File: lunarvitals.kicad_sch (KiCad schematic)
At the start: 29 parts, among them J1 MLX90614, J2 MAX30102, J3 SEN11574, J4 ConductiveCord, U1 NRF52840-DONGLE, U2 BMP280, U3 AP2112K-3.3, U5 MPU-6050

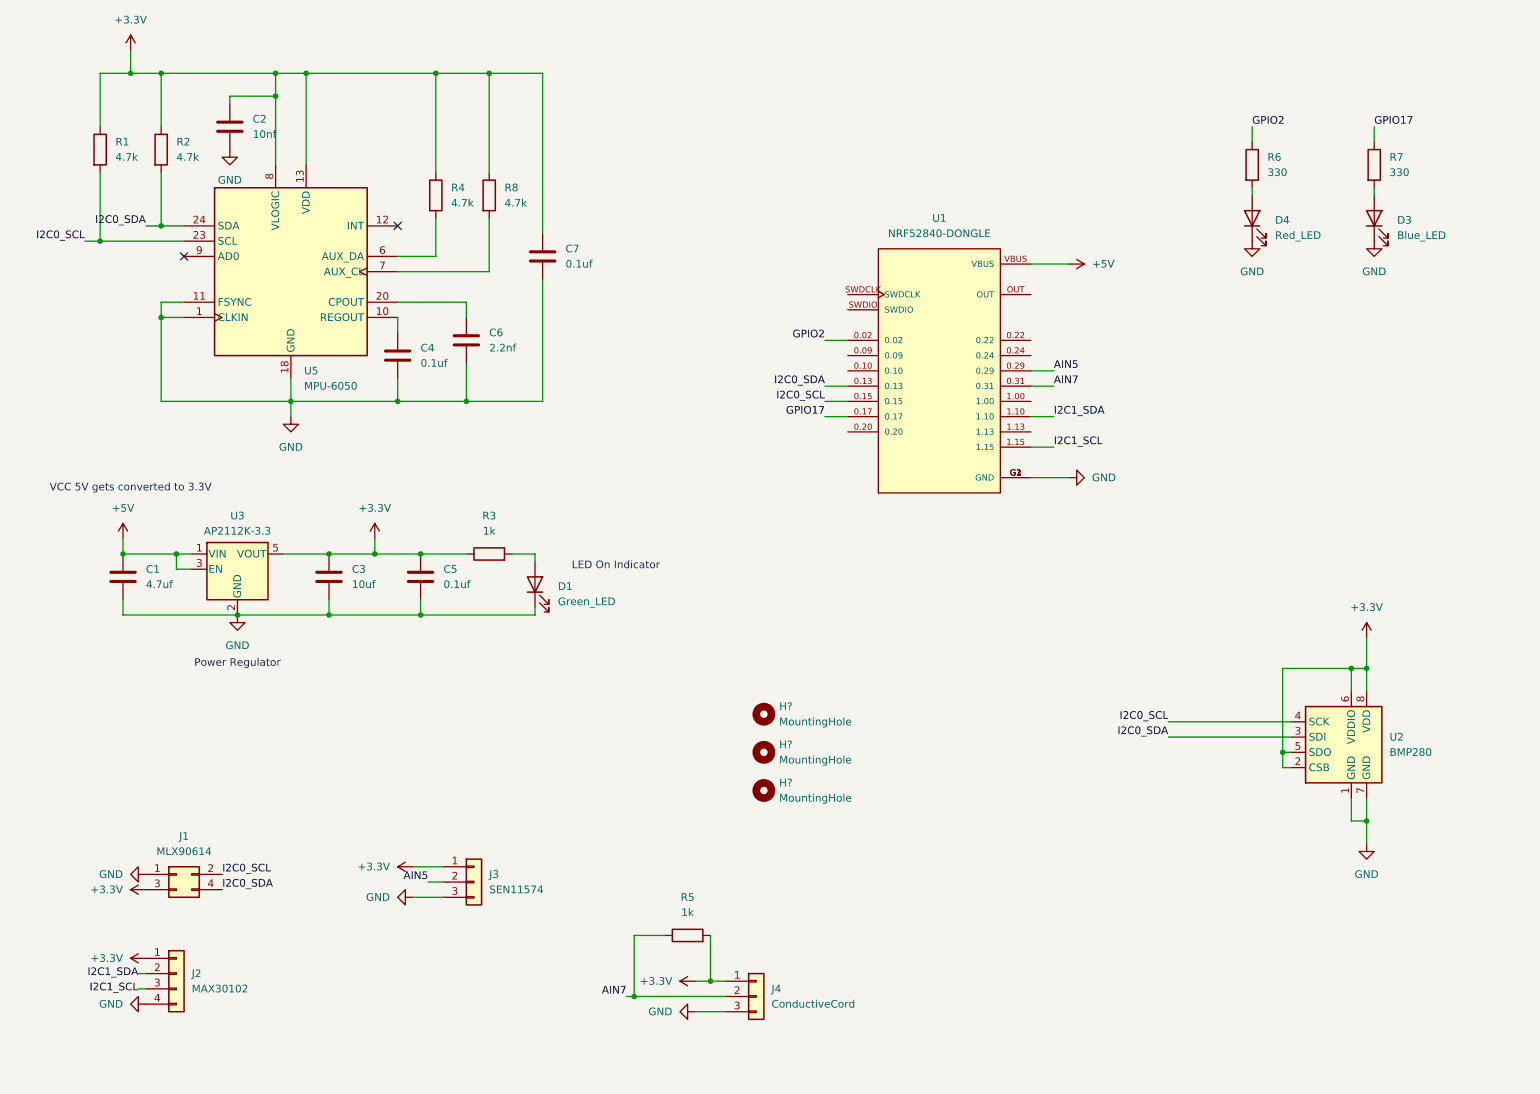
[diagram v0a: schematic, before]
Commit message: PCB Updates
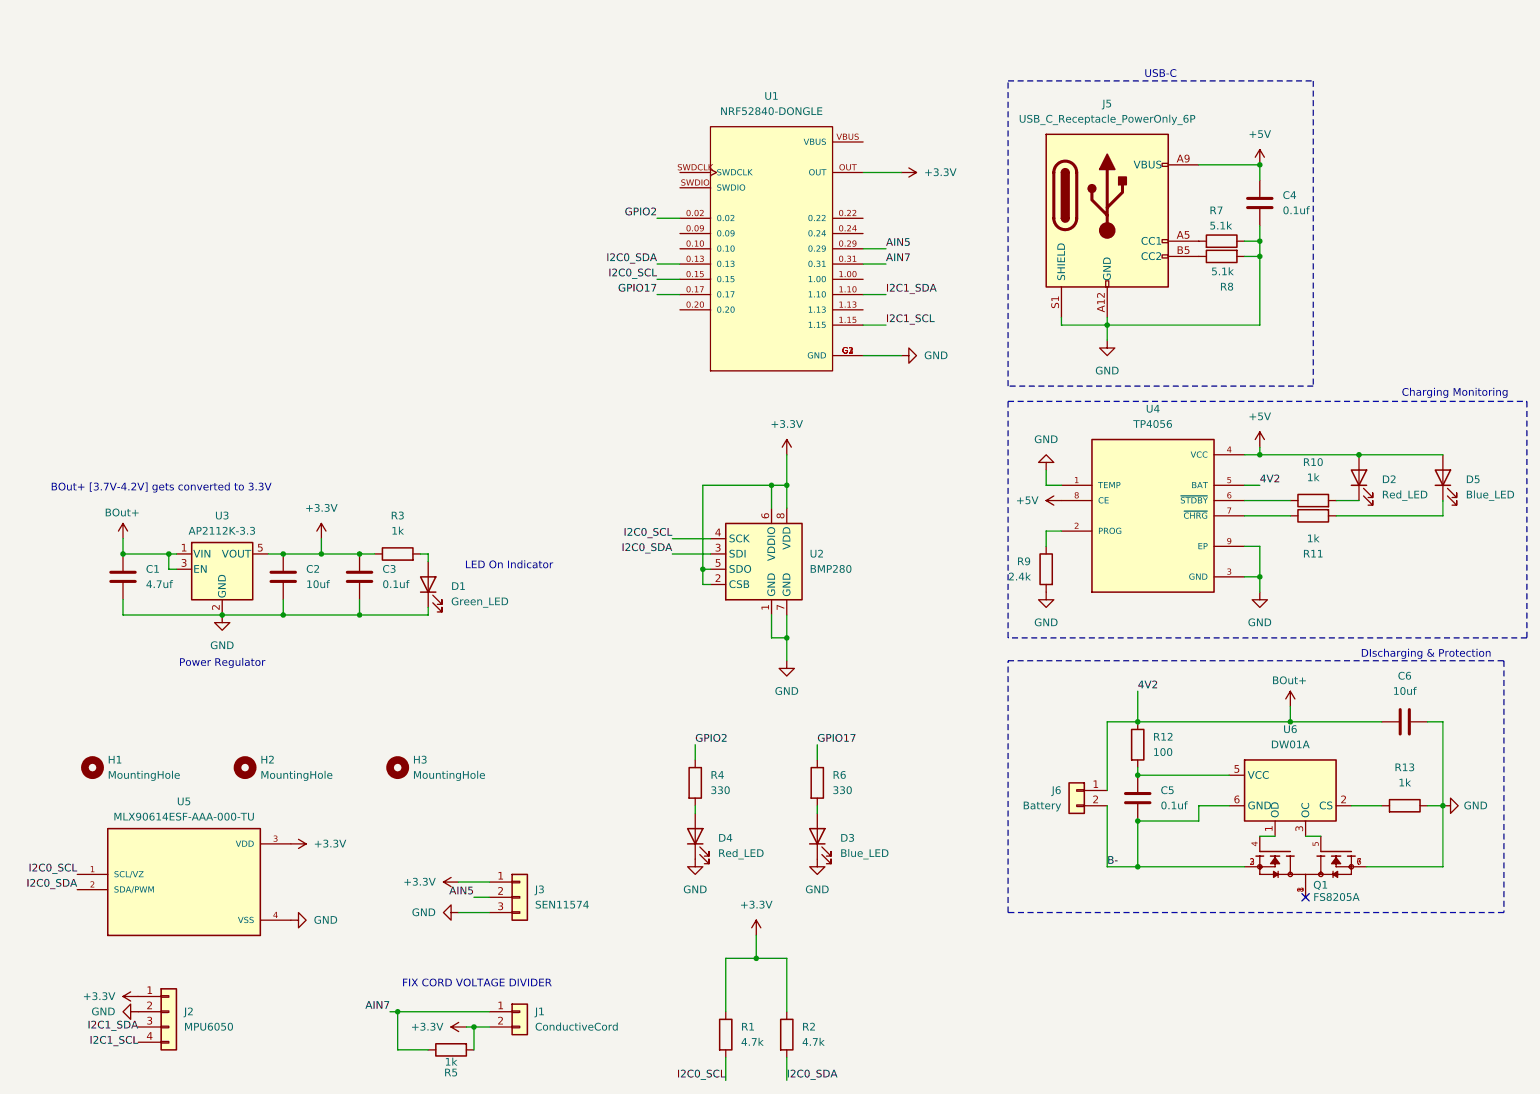
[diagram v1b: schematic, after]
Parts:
- removed C7: 0.1uf, Capacitor_SMD:C_0402_1005Metric, symbol Device:C
- removed J1: MLX90614, Connector_PinSocket_2.00mm:PinSocket_2x02_P2.00mm_Vertical, symbol Connector_Generic:Conn_02x02_Odd_Even
- removed J4: ConductiveCord, Connector_JST:JST_XA_B03B-XASK-1-A_1x03_P2.50mm_Vertical, symbol Connector_Generic:Conn_01x03
- removed U5: MPU-6050, Sensor_Motion:InvenSense_QFN-24_4x4mm_P0.5mm, symbol Sensor_Motion:MPU-6050
- added D2: Red_LED, LED_SMD:LED_0603_1608Metric, symbol Device:LED
- added D5: Blue_LED, LED_SMD:LED_0603_1608Metric, symbol Device:LED
- added J1: ConductiveCord, Connector_JST:JST_XH_B2B-XH-AM_1x02_P2.50mm_Vertical, symbol Connector_Generic:Conn_01x02
- added J5: USB_C_Receptacle_PowerOnly_6P, Connector_USB:USB_C_Receptacle_GCT_USB4125-xx-x-0190_6P_TopMnt_Horizontal, symbol Connector:USB_C_Receptacle_PowerOnly_6P
- added J6: Battery, SM02B-SRSS-TB_LF__SN_:SM02B-SRSS-TB_LF__SN_, symbol Connector_Generic:Conn_01x02
- added Q1: FS8205A, FS8205A:SOP65P640X120-8N, symbol FS8205A:FS8205A
- added R10, R11, R13: 1k, Resistor_SMD:R_0402_1005Metric, symbol Device:R
- added R12: 100, Resistor_SMD:R_0402_1005Metric, symbol Device:R
- added R9: 2.4k, Resistor_SMD:R_0402_1005Metric, symbol Device:R
- added U4: TP4056, TP4056:SOP127P600X175-9N, symbol TP4056:TP4056
- added U5: MLX90614ESF-AAA-000-TU, MLX90614ESF-AAA-000-TU:TO254P912H435-4, symbol MLX90614:MLX90614ESF-AAA-000-TU
- added U6: DW01A, Package_TO_SOT_SMD:SOT-23-6, symbol Battery_Management:DW01A
- C2: value 10nf -> 10uf; LCSC C1524 -> C15525
- C3: value 10uf -> 0.1uf; LCSC C15525 -> C1525
- C6: value 2.2nf -> 10uf; LCSC C1531 -> C15525
- J2: value MAX30102 -> MPU6050; footprint Connector_JST:JST_XA_B04B-XASK-1-A_1x04_P2.50mm_Vertical -> Connector_JST:JST_XH_B4B-XH-AM_1x04_P2.50mm_Vertical
- J3: footprint Connector_JST:JST_XA_B03B-XASK-1-A_1x03_P2.50mm_Vertical -> Connector_JST:JST_XH_B3B-XH-AM_1x03_P2.50mm_Vertical
- R4: value 4.7k -> 330; LCSC C25900 -> C12246
- R7: value 330 -> 5.1k; LCSC C12246 -> C25905
- R8: value 4.7k -> 5.1k; LCSC C25900 -> C25905
- gave numbers to parts that had none: 3
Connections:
- net +3.3V: now also U1.OUT, J1.2 (Pin_2), U5.3 (VDD); no longer C5.1, R4.1, R8.1
- net +5V: now also C4.1, D2.2 (A), D5.2 (A), J5.A9 (VBUS), J5.B9 (VBUS), U4.4 (VCC), U4.8 (CE); no longer C1.1, U1.VBUS, U3.1 (VIN), U3.3 (EN)
- net AIN7: now also J1.1 (Pin_1)
- net GND: now also J2.2 (Pin_2), R7.1, R8.2, J5.A12 (GND), J5.B12 (GND), J5.S1 (SHIELD), Q1.6, Q1.7, R13.1, R9.2, U4.1 (TEMP), U4.3 (GND), U4.9 (EP), U5.4 (VSS); no longer C5.2, J2.4 (Pin_4)
- net GPIO17: now also R6.1; no longer R7.1
- net GPIO2: now also R4.1; no longer R6.1
- net I2C0_SCL: now also U5.1 (SCL/VZ)
- net I2C0_SDA: now also U5.2 (SDA/PWM)
- net I2C1_SCL: now also J2.4 (Pin_4); no longer J2.3 (Pin_3)
- net I2C1_SDA: now also J2.3 (Pin_3); no longer J2.2 (Pin_2)
- net BOut+: now reaches C6.1
- net BOut+: now also C1.1, U3.1 (VIN), U3.3 (EN), J6.1 (Pin_1), R12.1, U4.5 (BAT)
- net at R4.2: now also D4.2 (A)
- net at R6.2: now also D3.2 (A); no longer D4.2 (A)
- net at R7.2: now also J5.A5 (CC1); no longer D3.2 (A)
- new net: R9.1, U4.2 (PROG)
- new net: R10.1, U4.6 (~{STDBY})
- new net: D2.1 (K), R10.2
- new net: Q1.1, Q1.8
- new net: Q1.4, U6.1 (OD)
- new net: Q1.5, U6.3 (OC)
- new net: J5.B5 (CC2), R8.1
- new net: R11.1, U4.7 (~{CHRG})
- new net: D5.1 (K), R11.2
- new net: R13.2, U6.2 (CS)
- new net: C5.1, R12.2, U6.5 (VCC)
- new net B-: C5.2, J6.2 (Pin_2), Q1.2, Q1.3, U6.6 (GND)
- no-connect marks 2 -> 1
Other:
- note added: "BOut+ [3.7V-4.2V] gets converted to 3.3V"
- note added: "Charging Monitoring"
- note added: "DIscharging & Protection"
- note added: "FIX CORD VOLTAGE DIVIDER"
- note added: "USB-C"
- note removed: "VCC 5V gets converted to 3.3V"
- moved on the sheet: D1, D3, D4, H1, H2, H3, J2, J3, R3, R5, U1, U2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
